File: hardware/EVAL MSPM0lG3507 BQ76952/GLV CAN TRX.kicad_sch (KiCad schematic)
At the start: 14 parts, among them U10 MCP2542FDxMF, U15 AP63203WU, U5 ISO7721D

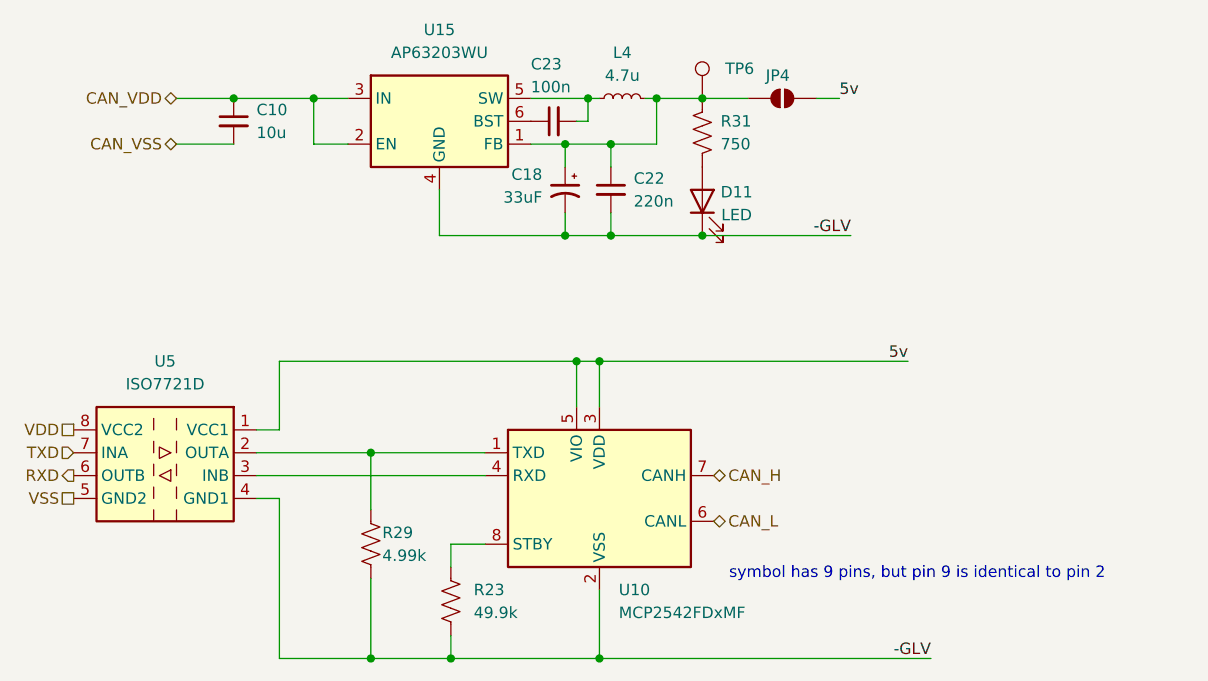
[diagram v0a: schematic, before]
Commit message: bluhhh
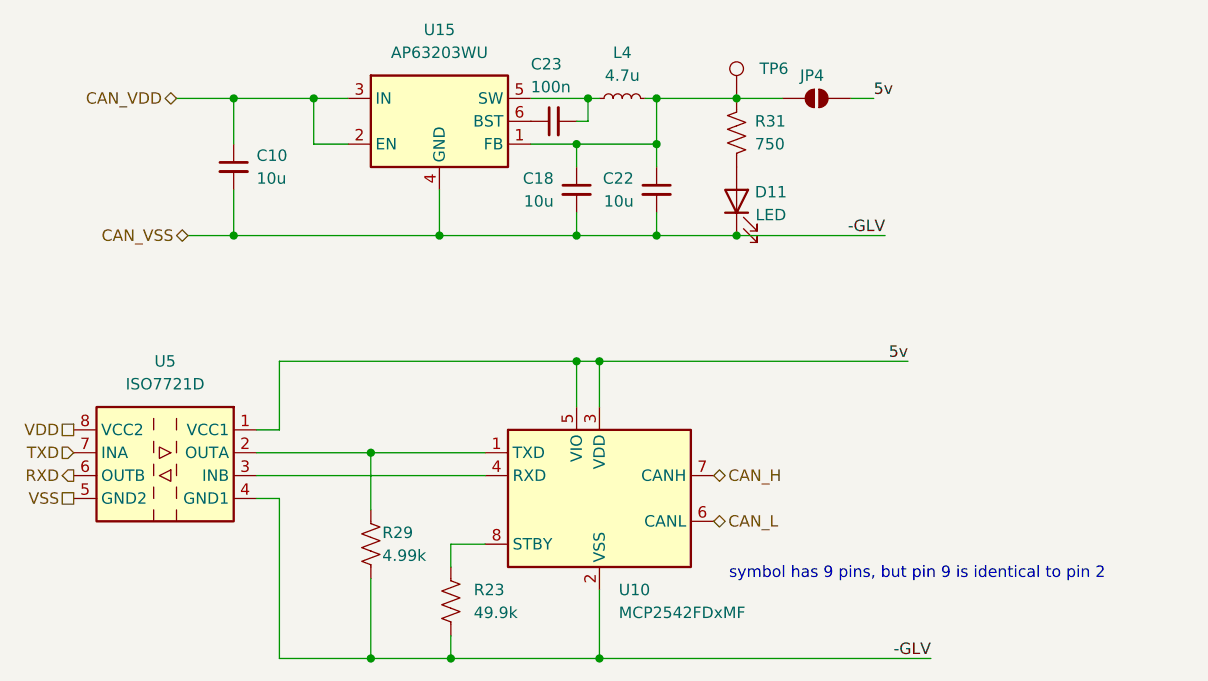
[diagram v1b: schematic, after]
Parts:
- removed C18: 33uF, Diode_SMD:D_1206_3216Metric_Pad1.42x1.75mm_HandSolder, symbol Device:C_Polarized_Small_US
- added C18: 10u, Capacitor_SMD:C_1206_3216Metric_Pad1.33x1.80mm_HandSolder, symbol Device:C_Small
- C22: value 220n -> 10u; mouser https://www.mouser.com/ProductDetail/Samsung-Electro-Mechanics/CL31B224KBFNNNF?qs=sGAEpiMZZMsh%252B1woXyUXj7iNKXiFkBmw7C%252BUlKpuDJ8%3D -> https://www.mouser.com/ProductDetail/Samsung-Electro-Mechanics/CL31A106KBHNNNE?qs=sGAEpiMZZMsh%252B1woXyUXjxqcB7t9naYpzWmpMbMJIKQ%3D; specs 50VDC, X7R, 10%, -55C, +125C, 220nF -> 10uF, 50VDC, X5R, 10%, -55C, +85C; unit x10 0.05 -> 0.07
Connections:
- net -GLV is gone; now on net CAN_VSS: C22.2, D11.1 (K), R23.1, R29.2, U10.2 (VSS), U10.9 (VSS), U15.4 (GND), U5.4 (GND1)
- net CAN_VSS: now also C18.2
- net at C22.1, JP4.1 (A), L4.2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: now also C18.1
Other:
- moved on the sheet: C10, D11, JP4, R31, TP6

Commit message: ac;lkacnl;
acea;kca
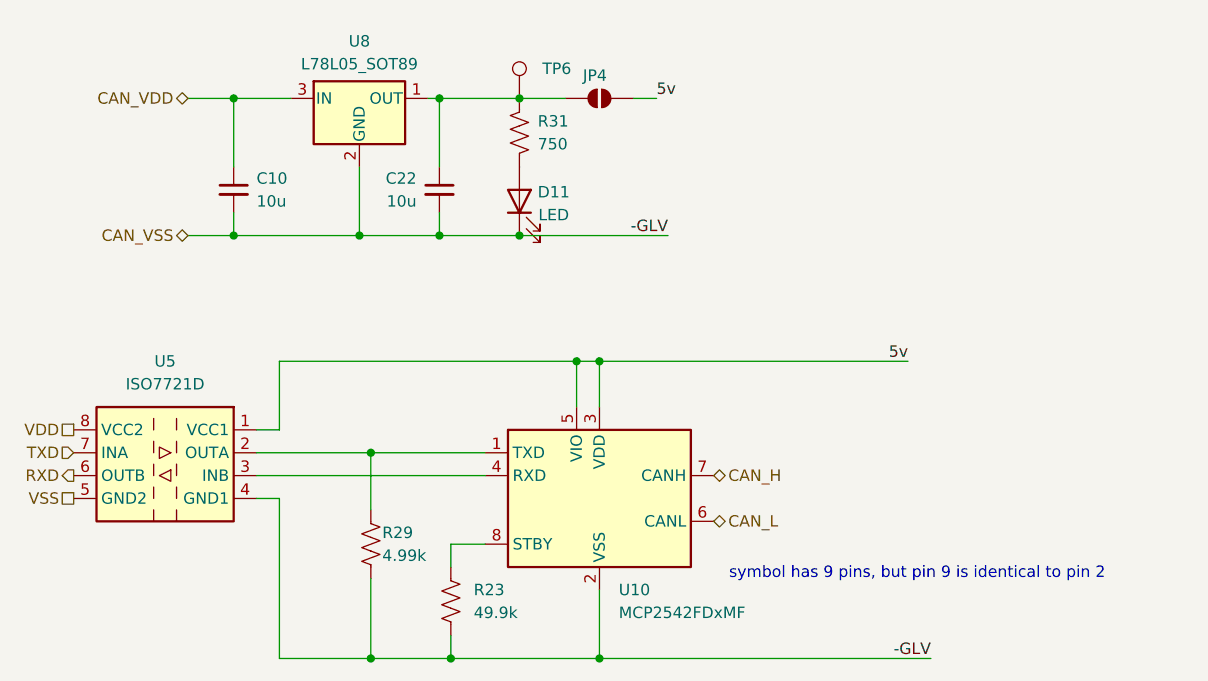
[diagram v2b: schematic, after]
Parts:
- removed C18: 10u, Capacitor_SMD:C_1206_3216Metric_Pad1.33x1.80mm_HandSolder, symbol Device:C_Small
- removed C23: 100n, Capacitor_SMD:C_1206_3216Metric_Pad1.33x1.80mm_HandSolder, symbol Device:C_Small
- removed L4: 4.7u, Inductor_SMD:L_0805_2012Metric_Pad1.05x1.20mm_HandSolder, symbol Device:L_Small
- removed U15: AP63203WU, Package_TO_SOT_SMD:TSOT-23-6, symbol Regulator_Switching:AP63203WU
- added U8: L78L05_SOT89, Package_TO_SOT_SMD:SOT-89-3, symbol Regulator_Linear:L78L05_SOT89
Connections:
- net CAN_VDD: now also U8.3 (IN)
- net CAN_VSS: now also U8.2 (GND)
- net at C22.1, JP4.1 (A), R31.1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: now also U8.1 (OUT)
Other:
- moved on the sheet: C10, C22, D11, JP4, R31, TP6
